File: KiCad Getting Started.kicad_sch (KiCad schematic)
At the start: 0 parts

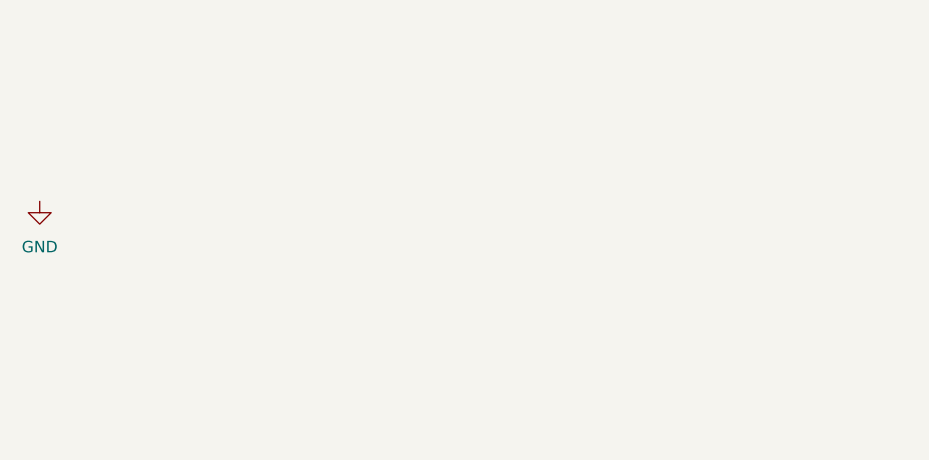
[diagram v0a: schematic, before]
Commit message: Schematic Tutorial
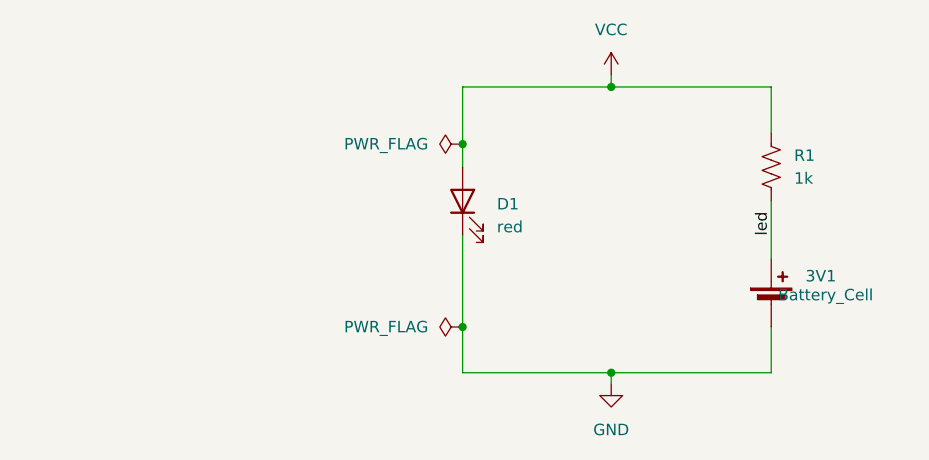
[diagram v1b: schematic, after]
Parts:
- added 3V1: Battery_Cell, Battery:BatteryHolder_Keystone_1058_1x2032, symbol Device:Battery_Cell
- added D1: red, LED_THT:LED_D5.0mm, symbol Device:LED
- added R1: 1k, Resistor_THT:R_Axial_DIN0309_L9.0mm_D3.2mm_P12.70mm_Horizontal, symbol Device:R_US
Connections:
- net GND: now also 3V1.2 (-), D1.1 (K)
- new net VCC: D1.2 (A), R1.2
- new net led: 3V1.1 (+), R1.1
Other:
- title: (none) -> Getting Started

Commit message: Done!
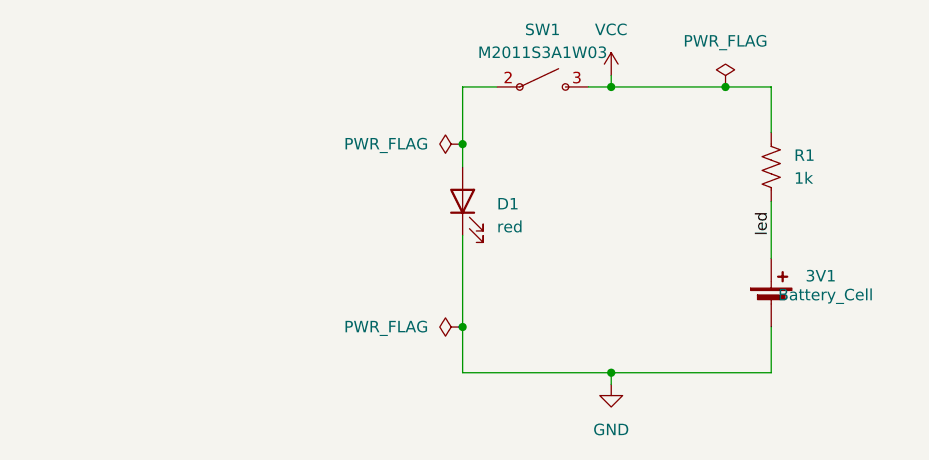
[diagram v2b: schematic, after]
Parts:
- added SW1: M2011S3A1W03, getting-started:Switch_Toggle_SPST_NKK_M2011S3A1x03, symbol getting-started:M2011S3A1W03
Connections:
- net VCC: now also SW1.3 (B); no longer D1.2 (A)
- new net: D1.2 (A), SW1.2 (A)
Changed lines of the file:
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@@
+	)
+	(junction
+		(at 182.88 81.28)
+		(diameter 0)
+		(color 0 0 0 0)
 	)
 	(junction
@@
 	(wire
 		(pts
-			(xy 170.18 81.28) (xy 153.67 81.28)
-		)
-		(stroke
-			(width 0)
-			(type default)
-		)
-	)
-	(wire
-		(pts
 			(xy 153.67 81.28) (xy 153.67 87.63)
 		)
@@
 	(wire
 		(pts
+			(xy 153.67 81.28) (xy 157.48 81.28)
+		)
+		(stroke
+			(width 0)
+			(type default)
+		)
+	)
+	(wire
+		(pts
+			(xy 182.88 81.28) (xy 170.18 81.28)
+		)
+		(stroke
+			(width 0)
+			(type default)
+		)
+	)
+	(wire
+		(pts
 			(xy 187.96 113.03) (xy 187.96 107.95)
 		)
@@
 	(wire
 		(pts
-			(xy 187.96 81.28) (xy 170.18 81.28)
+			(xy 167.64 81.28) (xy 170.18 81.28)
+		)
+		(stroke
+			(width 0)
+			(type default)
+		)
+	)
+	(wire
+		(pts
+			(xy 187.96 81.28) (xy 182.88 81.28)
 		)
 		(stroke
@@
 	)
 	(symbol
+		(lib_id "power:PWR_FLAG")
+		(at 182.88 81.28 0)
+		(unit 1)
+		(body_style 1)
+		(exclude_from_sim no)
+		(in_bom yes)
+		(on_board yes)
+		(in_pos_files yes)
+		(dnp no)
+		(fields_autoplaced yes)
+		(property "Reference" "#FLG03"
+			(at 182.88 79.375 0)
+			(hide yes)
+			(show_name no)
+			(do_not_autoplace no)
+			(effects
+				(font
+					(size 1.27 1.27)
+				)
+			)
+		)
+		(property "Value" "PWR_FLAG"
+			(at 182.88 76.2 0)
+			(show_name no)
+			(do_not_autoplace no)
+			(effects
+				(font
+					(size 1.27 1.27)
+				)
+			)
+		)
+		(property "Footprint" ""
+			(at 182.88 81.28 0)
+			(hide yes)
+			(show_name no)
+			(do_not_autoplace no)
+			(effects
+				(font
+					(size 1.27 1.27)
+				)
+			)
+		)
+		(property "Datasheet" ""
+			(at 182.88 81.28 0)
+			(hide yes)
+			(show_name no)
+			(do_not_autoplace no)
+			(effects
+				(font
+					(size 1.27 1.27)
+				)
+			)
+		)
+		(property "Description" "Special symbol for telling ERC where power comes from"
+			(at 182.88 81.28 0)
+			(hide yes)
+			(show_name no)
+			(do_not_autoplace no)
+			(effects
+				(font
+					(size 1.27 1.27)
+				)
+			)
+		)
+		(pin "1"
+		)
+		(instances
+			(project "KiCad Getting Started"
+				(path "/9cc72b08-ad7d-4d97-baba-2379e1bd8e58"
+					(reference "#FLG03")
+					(unit 1)
+				)
+			)
+		)
+	)
+	(symbol
 		(lib_id "power:VCC")
 		(at 170.18 80.01 0)
@@
 					(unit 1)
 				)
+			)
+		)
+	)
+	(symbol
+		(lib_id "getting-started:M2011S3A1W03")
+		(at 162.56 81.28 0)
+		(unit 1)
+		(body_style 1)
+		(exclude_from_sim no)
+		(in_bom yes)
+		(on_board yes)
+		(in_pos_files yes)
+		(dnp no)
+		(fields_autoplaced yes)
+		(property "Reference" "SW1"
+			(at 162.56 74.93 0)
+			(show_name no)
+			(do_not_autoplace no)
+			(effects
+				(font
+					(size 1.27 1.27)
+				)
+			)
+		)
+		(property "Value" "M2011S3A1W03"
+			(at 162.56 77.47 0)
+			(show_name no)
+			(do_not_autoplace no)
+			(effects
+				(font
+					(size 1.27 1.27)
+				)
+			)
+		)
+		(property "Footprint" "getting-started:Switch_Toggle_SPST_NKK_M2011S3A1x03"
+			(at 162.56 81.28 0)
+			(hide yes)
+			(show_name no)
+			(do_not_autoplace no)
+			(effects
+				(font
+					(size 1.27 1.27)
+				)
+			)
+		)
+		(property "Datasheet" ""
+			(at 162.56 81.28 0)
+			(hide yes)
+			(show_name no)
+			(do_not_autoplace no)
+			(effects
+				(font
+					(size 1.27 1.27)
+				)
+			)
+		)
+		(property "Description" ""
+			(at 162.56 81.28 0)
+			(hide yes)
+			(show_name no)
+			(do_not_autoplace no)
+			(effects
+				(font
+					(size 1.27 1.27)
+				)
+			)
+		)
+		(pin "2"
+		)
+		(pin "3"
+		)
+		(instances
+			(project "KiCad Getting Started"
+				(path "/9cc72b08-ad7d-4d97-baba-2379e1bd8e58"
+					(reference "SW1")
+					(unit 1)
+				)
